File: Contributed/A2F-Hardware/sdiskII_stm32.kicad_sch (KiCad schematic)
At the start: 32 parts, among them J1 SDISKII IN (CARD), J2 SDISKII OUT (DRIVE), J3 EA W128064-OLED (FPC31), J4 UART, U1 BlackPill STMF4X1, U2 DM-OLED096-636, U3 EA OLEDM128-6, U4 74x257

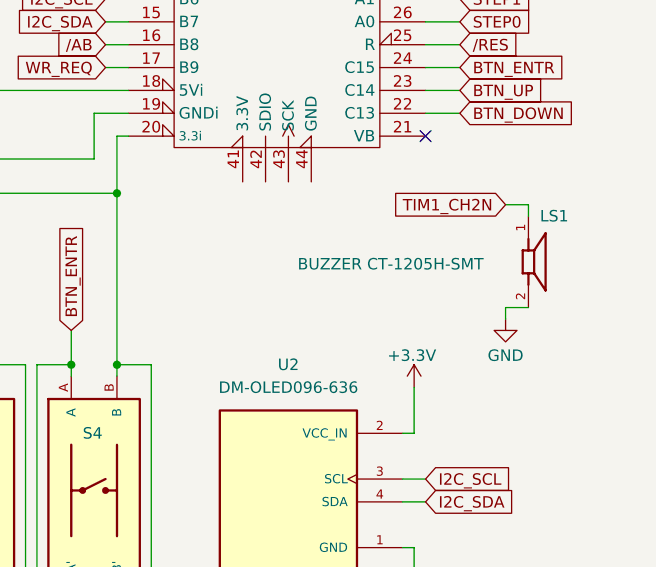
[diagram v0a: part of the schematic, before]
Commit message: RE update
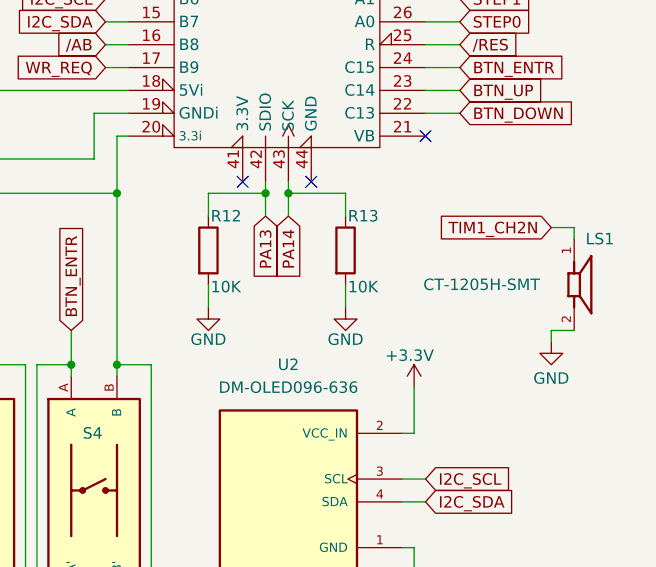
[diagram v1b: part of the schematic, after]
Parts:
- added R12, R13: 10K, Resistor_SMD:R_0805_2012Metric_Pad1.20x1.40mm_HandSolder, symbol Device:R
- LS1: value BUZZER CT-1205H-SMT -> CT-1205H-SMT
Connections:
- net GND: now also R12.2, R13.2
- net PA13: now also U1.42 (SDIO), R12.1
- net PA14: now also U1.43 (SCK), R13.1
- no-connect marks 16 -> 18
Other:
- moved on the sheet: LS1

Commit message: Make Filsystem fixed
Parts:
- U1: footprint acheron_Hardware.pretty-master:Mini_F4X1_STM32_VIB -> sdisk_stm32:Mini_F4X1_STM32_VIB
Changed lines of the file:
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@@
 (kicad_sch
-	(version 20231120)
+	(version 20250114)
 	(generator "eeschema")
-	(generator_version "8.0")
+	(generator_version "9.0")
 	(paper "A4")
 	(title_block
@@
 		(rev "20")
 	)
+	(rectangle
+		(start 132.08 60.96)
+		(end 176.53 102.87)
+		(stroke
+			(width 0)
+			(type default)
+		)
+		(fill
+			(type none)
+		)
+	)
+	(text "ALPS Rotary Encoder"
+		(exclude_from_sim no)
+		(at 155.702 63.754 0)
+		(effects
+			(font
+				(size 1.27 1.27)
+			)
+		)
+	)
 	(junction
 		(at 207.01 114.3)
@@
 		)
 	)
-	(rectangle
-		(start 132.08 60.96)
-		(end 176.53 102.87)
-		(stroke
-			(width 0)
-			(type default)
-		)
-		(fill
-			(type none)
-		)
-	)
-	(text "ALPS Rotary Encoder"
-		(exclude_from_sim no)
-		(at 155.702 63.754 0)
-		(effects
-			(font
-				(size 1.27 1.27)
-			)
-		)
-	)
 	(global_label "USART1_RX"
 		(shape input)
@@
 			)
 		)
-		(property "Footprint" "acheron_Hardware.pretty-master:Mini_F4X1_STM32_VIB"
+		(property "Footprint" "sdisk_stm32:Mini_F4X1_STM32_VIB"
 			(at 240.792 127.254 0)
 			(effects
@@
 		)
 	)
+	(embedded_fonts no)
 )
